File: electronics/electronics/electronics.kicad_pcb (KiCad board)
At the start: 2 copper layers, 21 parts, among them U1 TL071, U2 TL071, U3 TL071, U4 TL071

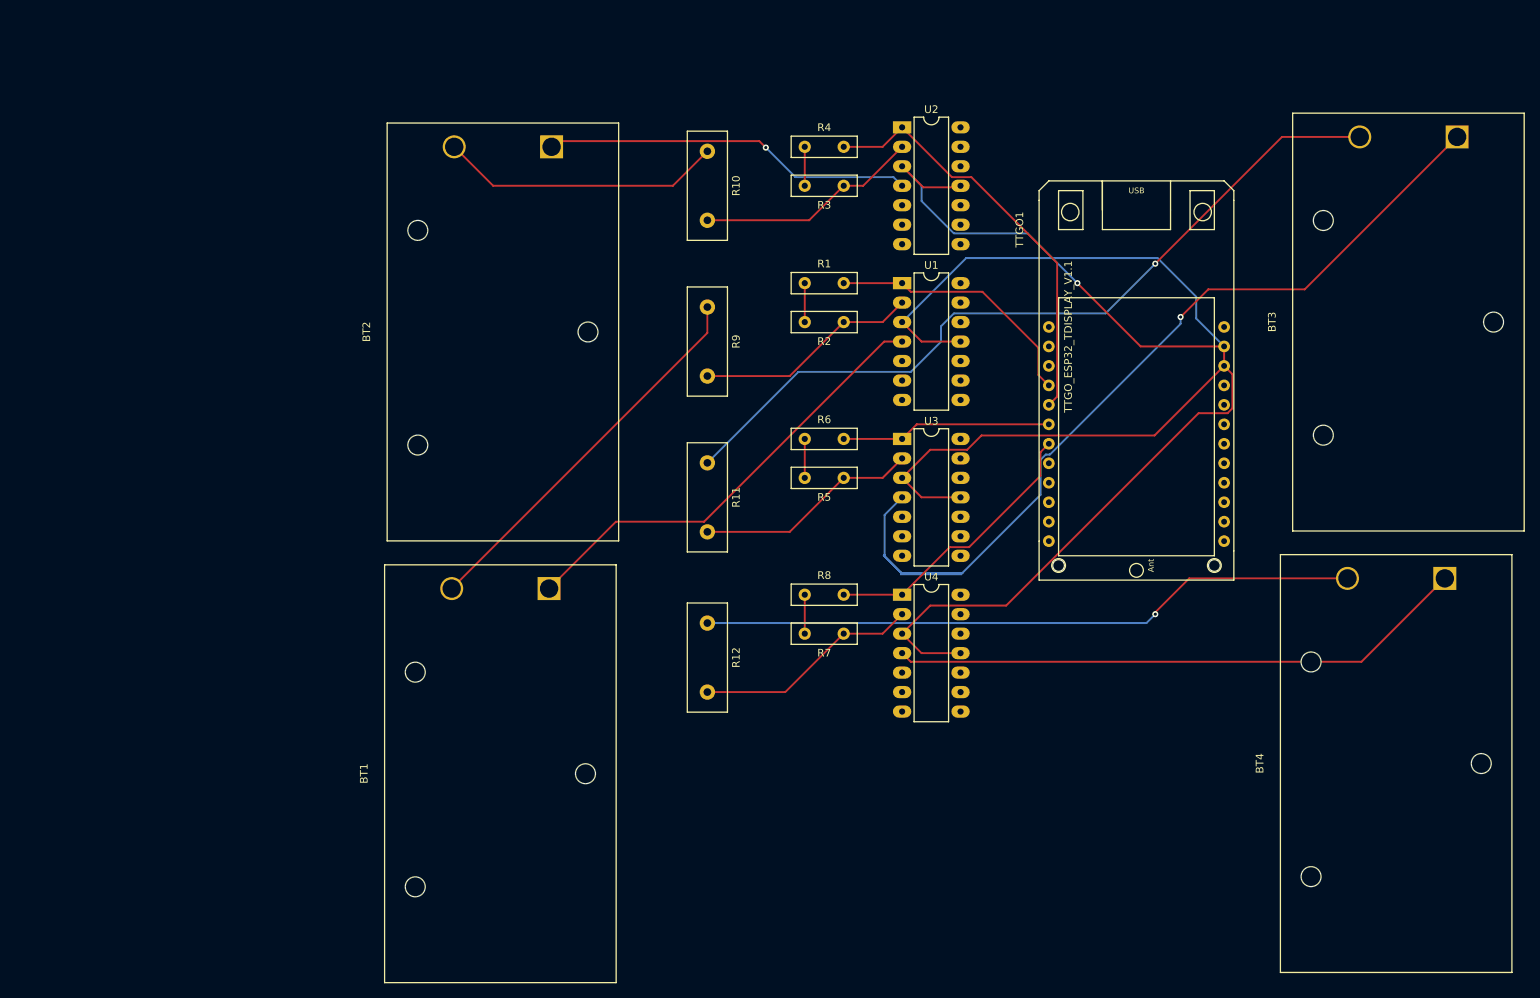
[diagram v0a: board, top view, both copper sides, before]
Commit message: kicad update
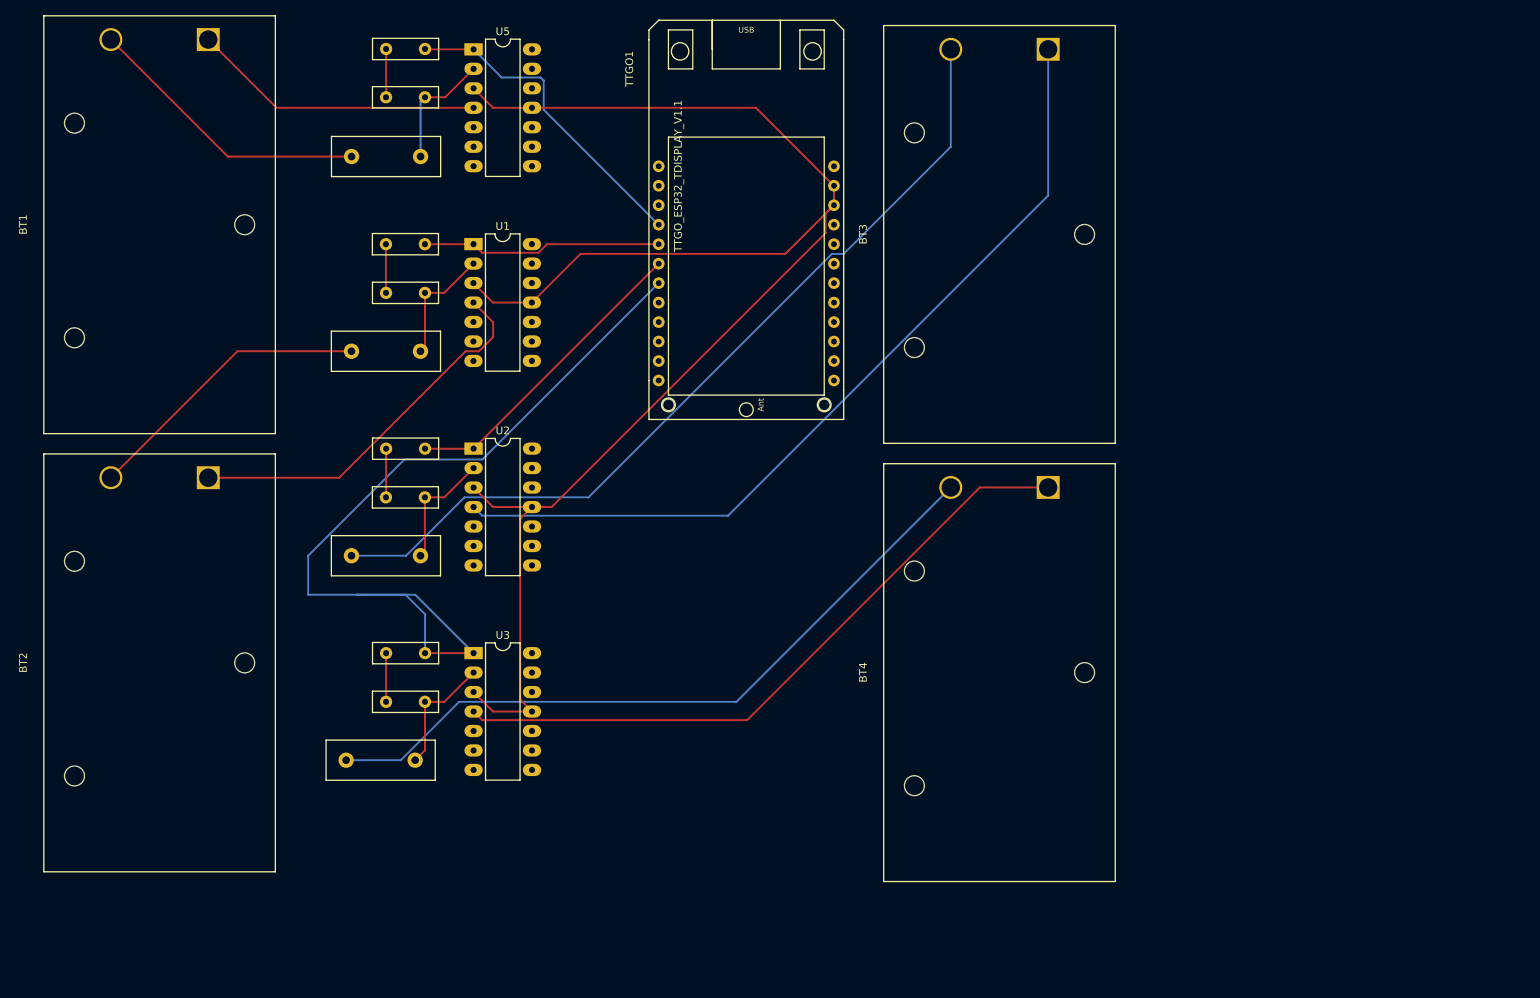
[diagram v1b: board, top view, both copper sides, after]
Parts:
- removed U4: TL071, Package_DIP:DIP-14_W7.62mm_LongPads
- added U5: TL074, Package_DIP:DIP-14_W7.62mm_LongPads, F.Cu at (71.1, 20.3)
- U1, U2, U3: value TL071 -> TL074
- moved BT1 84.3 mm to (36.5, 19.0)
- moved U2 69.9 mm to (71.1, 72.4)
- moved R1 62.6 mm to (59.7, 20.3)
- moved U3 62.5 mm to (71.1, 99.1)
- moved BT2 62.2 mm to (36.5, 76.2)
- moved R2 62.0 mm to (64.8, 26.6)
- moved R3 56.4 mm to (64.8, 52.1)
- moved U1 56.1 mm to (71.1, 45.7)
- moved R4 56.1 mm to (59.7, 45.7)
- moved R7 55.3 mm to (64.8, 105.4)
- moved R8 55.1 mm to (59.7, 99.1)
- moved TTGO1 55.0 mm to (94.0, 19.1)
- moved R5 54.7 mm to (64.8, 78.7)
- moved R6 54.6 mm to (59.7, 72.4)
- moved BT3 54.6 mm to (146.1, 20.3)
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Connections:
- BT1 pad 1: (no net) -> Net-(BT1-+)
- BT2 pad 1: (no net) -> Net-(BT2-+)
- BT3 pad 1: (no net) -> Net-(BT3-+)
- BT4 pad 1: (no net) -> Net-(BT4-+)
- R10 pad 2: Net-(U2A--) -> Net-(U1A--)
- R11 pad 2: Net-(U3A--) -> Net-(U2A--)
- R12 pad 2: Net-(U4A--) -> Net-(U3A--)
- R2 pad 1: Net-(U1A--) -> Net-(U5A--)
- R3 pad 1: Net-(U2A--) -> Net-(U1A--)
- R5 pad 1: Net-(U3A--) -> Net-(U2A--)
- R7 pad 1: Net-(U4A--) -> Net-(U3A--)
- R9 pad 2: Net-(U1A--) -> Net-(U5A--)
- U1 pad 1: Net-(TTGO1-GPIO26) -> Net-(TTGO1-GPIO25)
- U1 pad 4: (no net) -> Net-(BT2-+)
- U2 pad 1: Net-(TTGO1-GPIO25) -> Net-(TTGO1-GPIO33)
- U2 pad 4: (no net) -> Net-(BT3-+)
- U3 pad 1: Net-(TTGO1-GPIO33) -> Net-(TTGO1-GPIO32)
- U3 pad 4: (no net) -> Net-(BT4-+)
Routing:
- net (no net): track 306.1 -> 0.00 mm, vias 2 -> 0
- net Net-(BT3-+): track 0.00 -> 111.8 mm
- net Net-(BT4-+): track 0.00 -> 88.0 mm
- net Net-(TTGO1-GPIO32): track 36.7 -> 111.6 mm
- net Net-(BT2-+): track 0.00 -> 50.3 mm
- net Earth: track 251.8 -> 210.6 mm, vias 1 -> 0
- net Net-(BT1-+): track 0.00 -> 38.3 mm
- net Net-(U4A--): track 29.6 -> 0.00 mm
- net Net-(TTGO1-GPIO25): track 55.2 -> 31.4 mm
- net Net-(U5A--): track 0.00 -> 15.8 mm
- net Net-(U1A--): track 29.4 -> 15.8 mm
- net Net-(U2A--): track 29.4 -> 15.8 mm
- net Net-(U3A--): track 29.4 -> 16.1 mm
- net Net-(TTGO1-GPIO33): track 27.5 -> 40.5 mm
- net Net-(BT1--): track 50.5 -> 37.7 mm
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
